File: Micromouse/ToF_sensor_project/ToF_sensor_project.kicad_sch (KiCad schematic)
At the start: 6 parts, among them J3 Conn_01x03_Pin

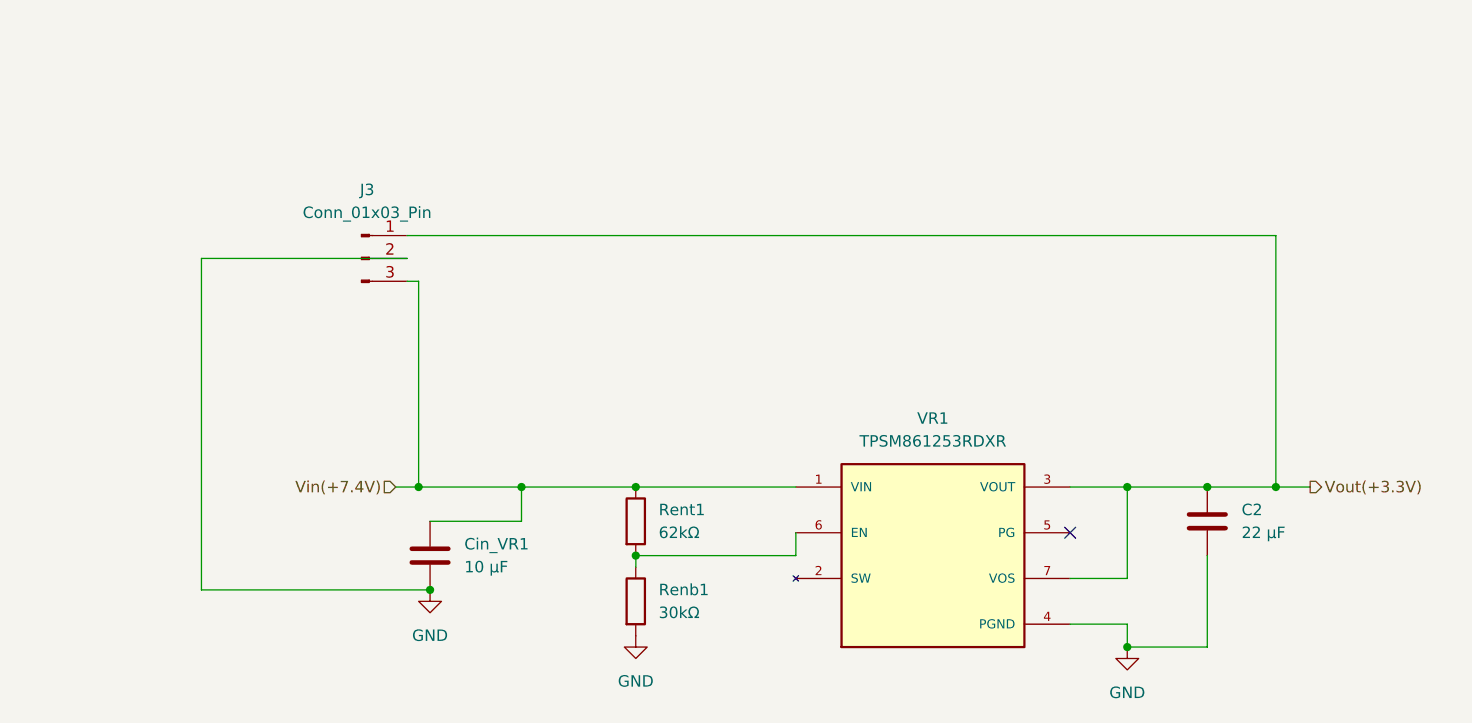
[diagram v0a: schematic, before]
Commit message: Schematic overhaul
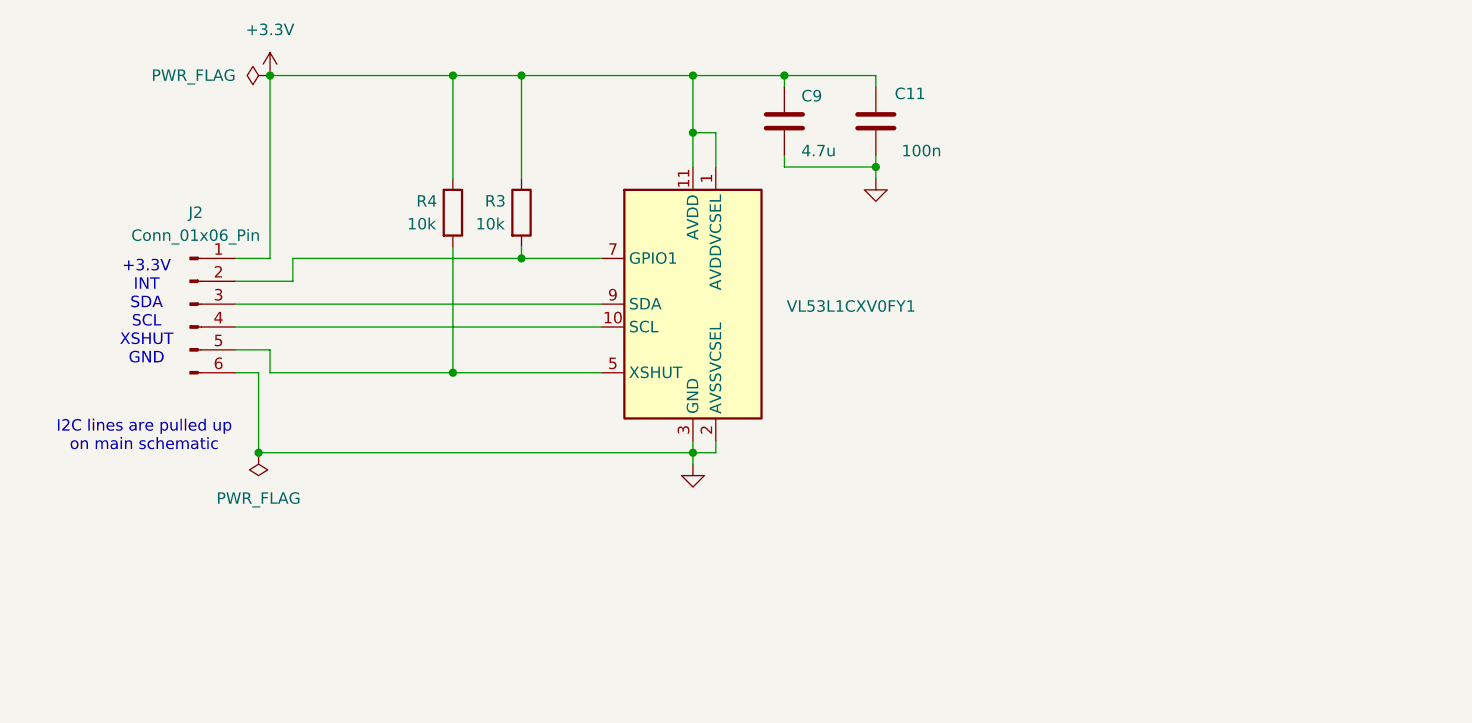
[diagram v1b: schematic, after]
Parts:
- removed C2: 22 µF, Capacitor_SMD:C_0402_1005Metric, symbol Device:C
- removed Cin_VR1: 10 µF, Capacitor_SMD:C_0402_1005Metric, symbol Device:C
- removed J3: Conn_01x03_Pin, Connector_JST:JST_ZH_B3B-ZR_1x03_P1.50mm_Vertical, symbol Connector:Conn_01x03_Pin
- removed Renb1: 30kΩ, Resistor_SMD:R_0603_1608Metric, symbol Device:R
- removed Rent1: 62kΩ, Resistor_SMD:R_0603_1608Metric, symbol Device:R
- removed VR1: TPSM861253RDXR, MM_TPSM861253RDXR:TPSM861253RDXR, symbol TPSM861253RDXR:TPSM861253RDXR
- added C11: 100n, Capacitor_SMD:C_0603_1608Metric, symbol Device:C
- added C9: 4.7u, Capacitor_SMD:C_0603_1608Metric, symbol Device:C
- added J2: Conn_01x06_Pin, symbol Connector:Conn_01x06_Pin
- added R3, R4: 10k, Resistor_SMD:R_0603_1608Metric, symbol Device:R
- added U1: VL53L1CXV0FY1, MM_VL53L4CDV0DH-1:LGA12_STM, symbol Sensor_Distance:VL53L1CXV0FY1
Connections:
- net GND: now also C11.1, C9.1, J2.6 (Pin_6), U1.12 (GND), U1.2 (AVSSVCSEL), U1.3 (GND), U1.4 (GND), U1.6 (GND)
- new net: J2.4 (Pin_4), U1.10 (SCL)
- new net: J2.5 (Pin_5), R4.2, U1.5 (XSHUT)
- new net: J2.2 (Pin_2), R3.2, U1.7 (GPIO1)
- new net: J2.3 (Pin_3), U1.9 (SDA)
- new net +3.3V: C11.2, C9.2, J2.1 (Pin_1), R3.1, R4.1, U1.1 (AVDDVCSEL), U1.11 (AVDD)
- no-connect marks 1 -> 0
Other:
- note added: "+3.3V INT SDA SCL XSHUT GND"
- note added: "I2C lines are pulled up on main schematic"
